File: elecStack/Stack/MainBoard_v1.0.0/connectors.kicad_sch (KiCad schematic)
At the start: 11 parts, among them J10 Conn_01x02_Socket, J2 Conn_01x06_Pin, J3 Conn_01x06_Pin, J4 Conn_01x02_Socket, J5 Conn_01x02_Socket, J6 Conn_01x07_Pin, J8 Conn_01x02_Socket, J9 Conn_01x02_Socket, U6 L293D

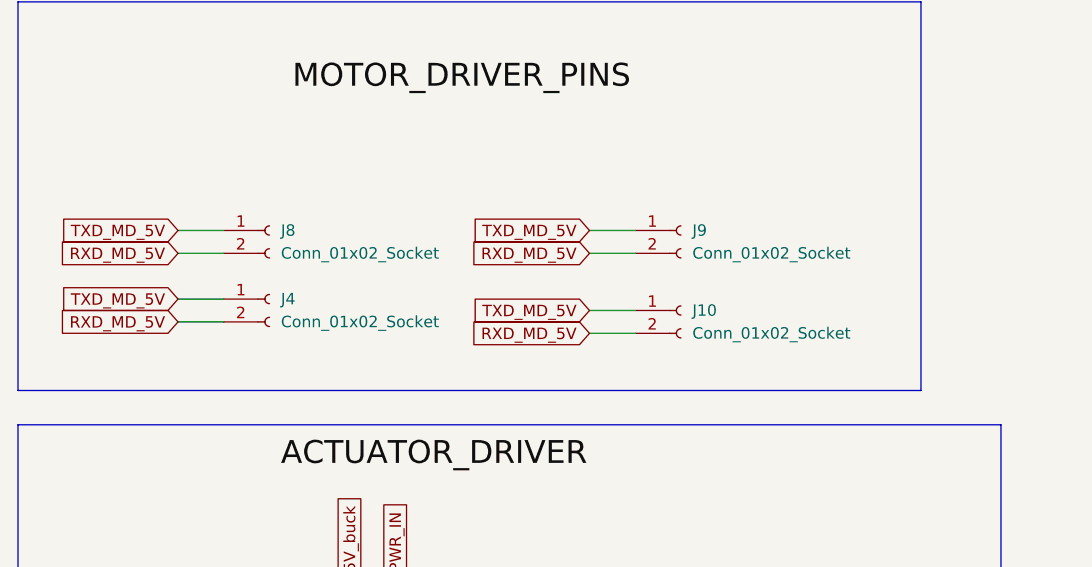
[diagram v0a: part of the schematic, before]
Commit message: version 1.2.0 layout done
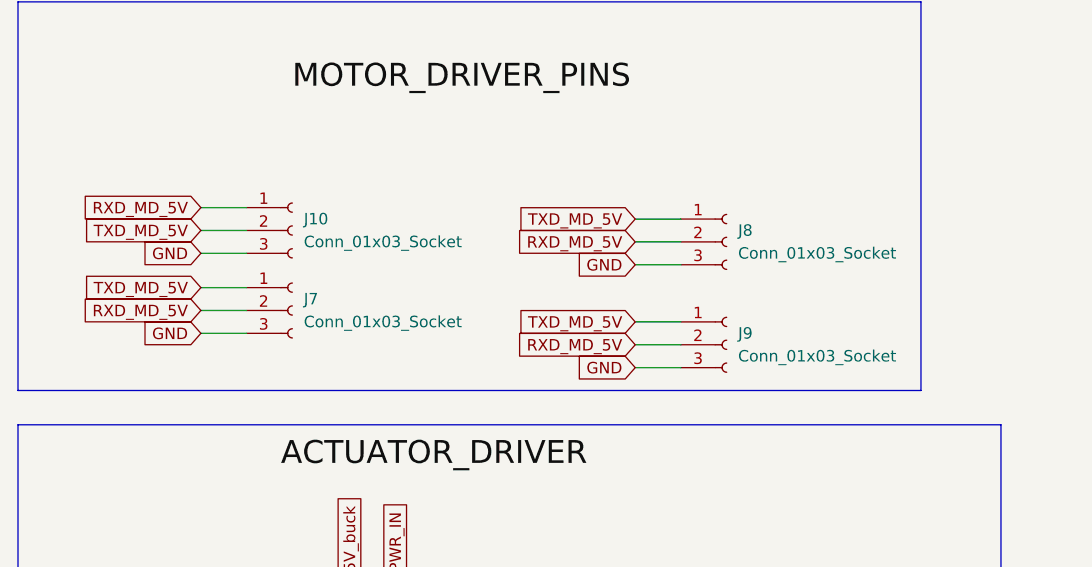
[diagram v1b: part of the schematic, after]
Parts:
- removed J10, J4, J8, J9: Conn_01x02_Socket, Connector_Phoenix_MSTB:PhoenixContact_MSTBA_2,5_2-G_1x02_P5.00mm_Horizontal, symbol Connector:Conn_01x02_Socket
- added J10, J7, J8, J9: Conn_01x03_Socket, Connector_JST:JST_EH_B3B-EH-A_1x03_P2.50mm_Vertical, symbol Connector:Conn_01x03_Socket
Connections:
- net GND: now also J10.3 (Pin_3), J7.3 (Pin_3), J8.3 (Pin_3), J9.3 (Pin_3)
- net RXD_MD_5V: now also J10.1 (Pin_1), J7.2 (Pin_2), J8.2 (Pin_2), J9.2 (Pin_2)
- net TXD_MD_5V: now also J10.2 (Pin_2), J7.1 (Pin_1), J8.1 (Pin_1), J9.1 (Pin_1)
